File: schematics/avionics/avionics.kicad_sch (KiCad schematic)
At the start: 15 parts, among them SW1 SW_SPST, SW2 SW_DPST, SW3 SW_SPST, SW4 SW_SPST, SW5 SW_DPST, U1 TeleMega

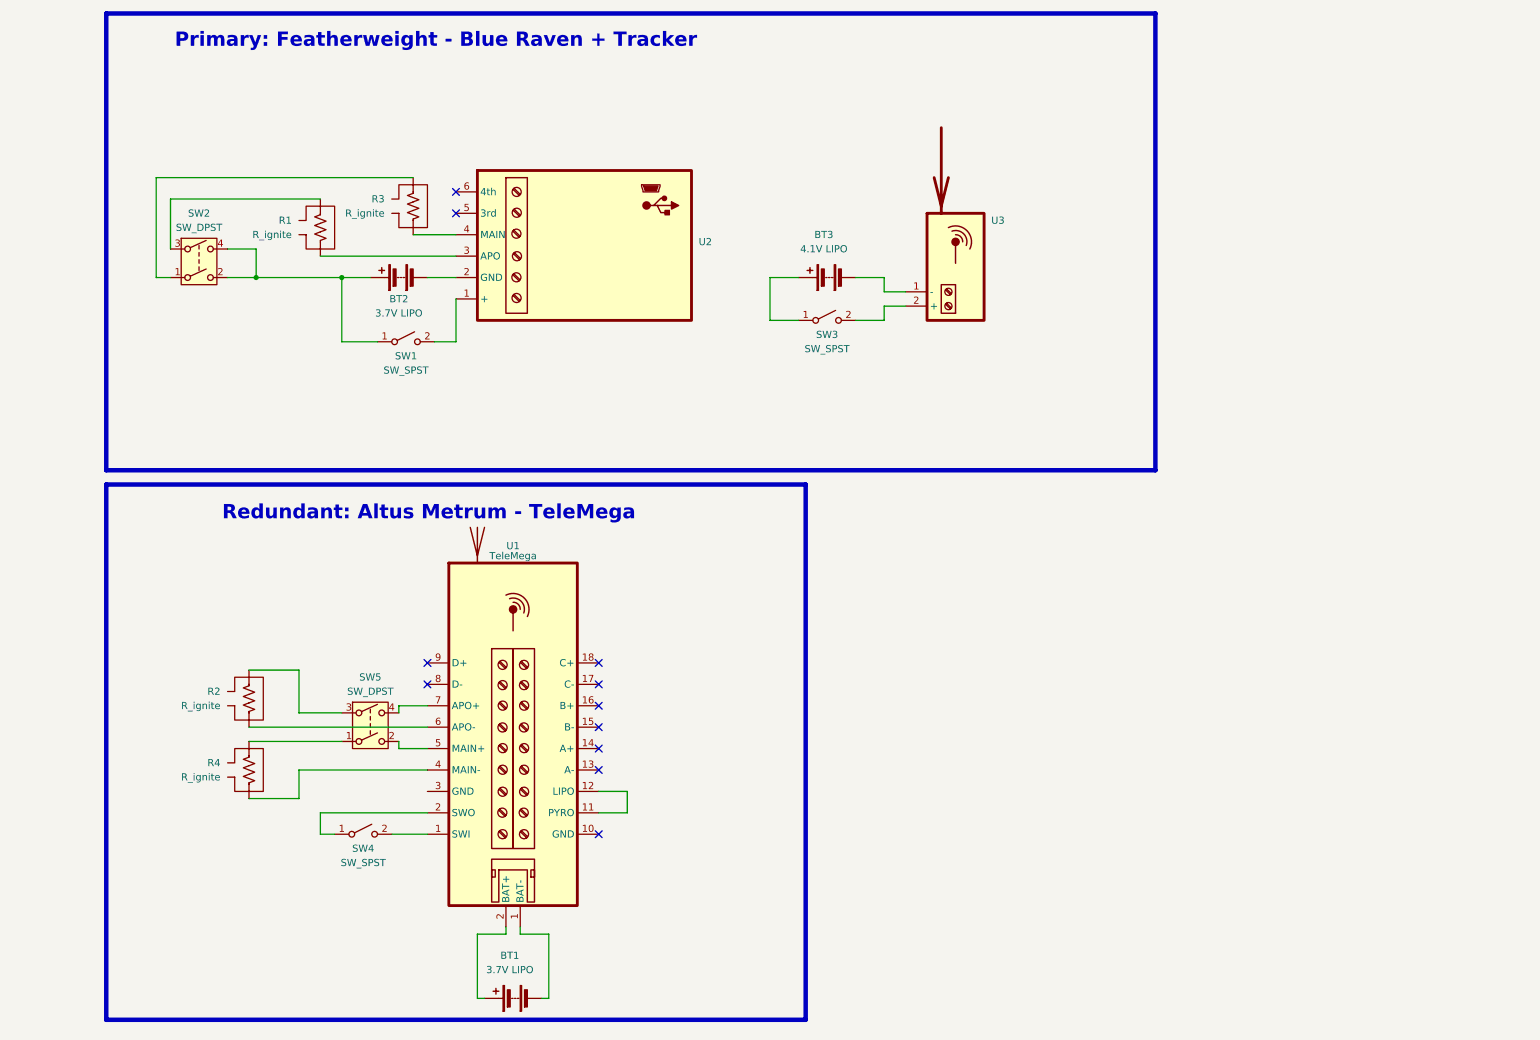
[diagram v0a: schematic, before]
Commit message: updated av bay schematic
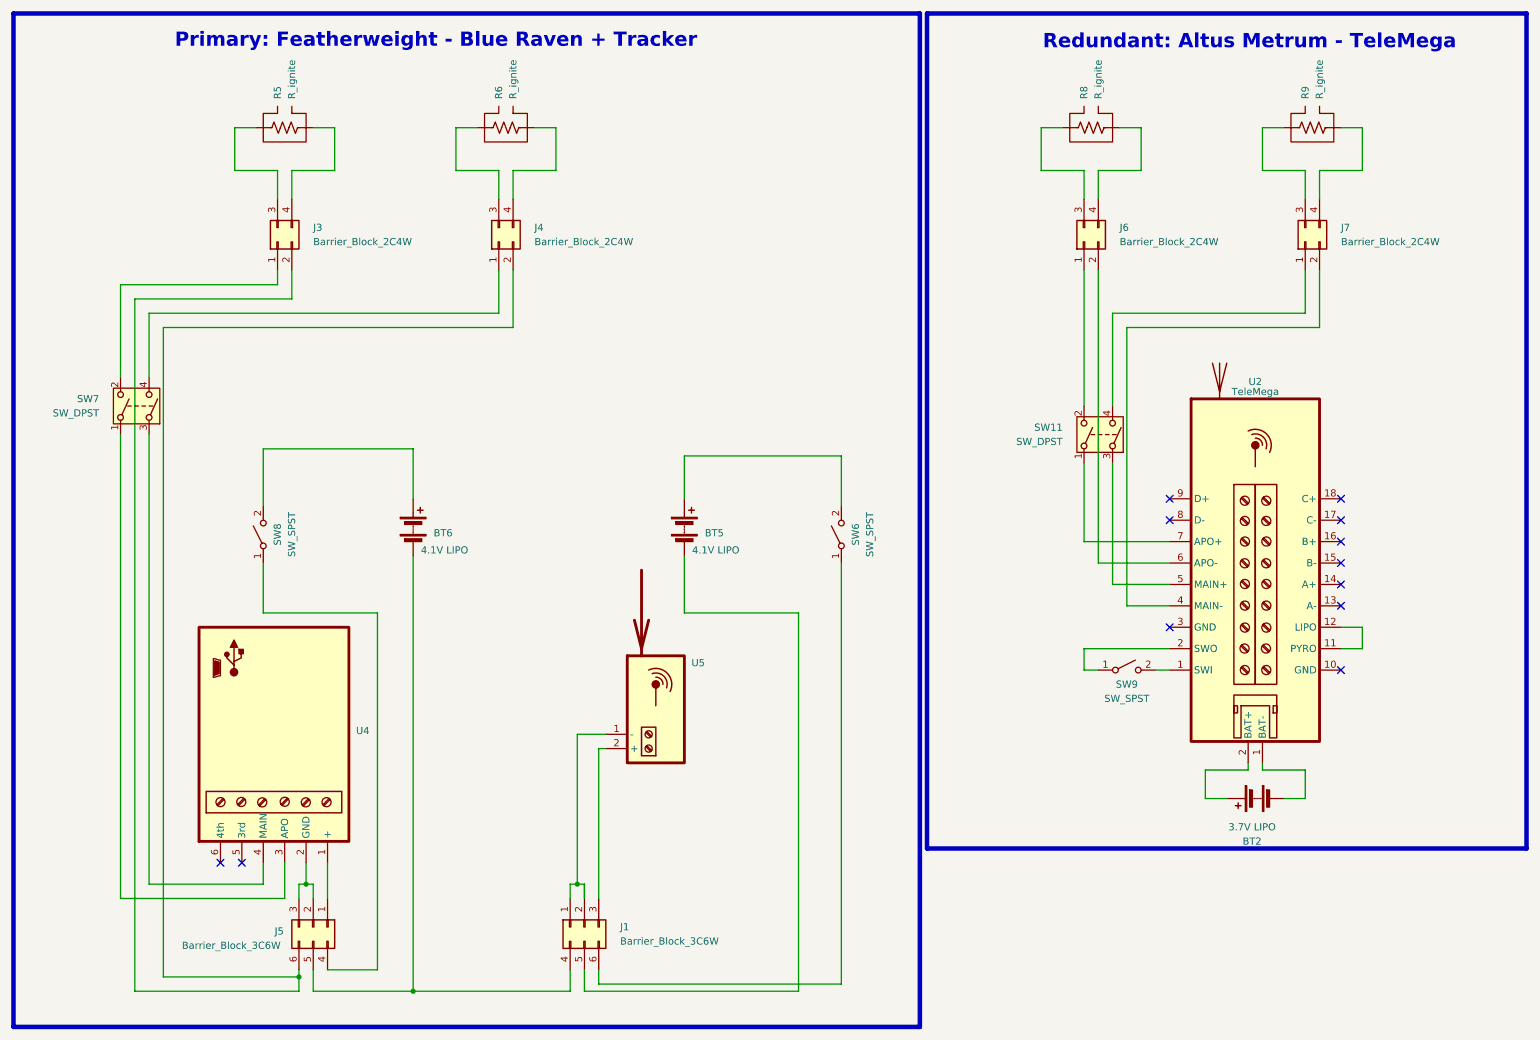
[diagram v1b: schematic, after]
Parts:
- removed BT1: 3.7V LIPO, symbol Device:Battery
- removed BT3: 4.1V LIPO, symbol Device:Battery
- removed R1, R2, R3, R4: R_ignite, symbol recovery:R_Igniter
- removed SW1, SW3, SW4: SW_SPST, symbol Switch:SW_SPST
- removed SW2, SW5: SW_DPST, symbol Switch:SW_DPST
- removed U1: TeleMega, symbol altusmetrum:telemega
- removed U2: ~, symbol featherweight:blue_raven
- removed U3: ~, symbol featherweight:tracker_gps
- added BT5, BT6: 4.1V LIPO, symbol Device:Battery
- added J1, J5: Barrier_Block_3C6W, symbol Connector_Generic:Conn_02x03_Top_Bottom
- added J3, J4, J6, J7: Barrier_Block_2C4W, symbol Connector_Generic:Conn_02x02_Top_Bottom
- added R5, R6, R8, R9: R_ignite, symbol recovery:R_Igniter
- added SW11, SW7: SW_DPST, symbol Switch:SW_DPST
- added SW6, SW8, SW9: SW_SPST, symbol Switch:SW_SPST
- added U2: TeleMega, symbol altusmetrum:telemega
- added U4: ~, symbol featherweight:blue_raven
- added U5: ~, symbol featherweight:tracker_gps
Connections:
- net at BT2.1 (+): now also U2.2 (BAT+)
- net at BT2.2 (-): now also U2.1 (BAT-)
- new net: BT5.1 (+), SW6.2 (B)
- new net: BT5.2 (-), J1.5 (Pin_5)
- new net: SW7.1, U4.3 (APO)
- new net: J3.1 (Pin_1), SW7.2
- new net: SW7.3, U4.4 (MAIN)
- new net: J4.1 (Pin_1), SW7.4
- new net: J3.2 (Pin_2), J4.2 (Pin_2), J5.6 (Pin_6)
- new net: J4.3 (Pin_3), R6.1
- new net: J4.4 (Pin_4), R6.2
- new net: SW9.1 (A), U2.2 (BAT+)
- new net: SW9.2 (B), U2.1 (BAT-)
- new net: J6.1 (Pin_1), SW11.2
- new net: J6.2 (Pin_2), U2.6 (APO-)
- new net: J6.3 (Pin_3), R8.1
- new net: J6.4 (Pin_4), R8.2
- new net: J5.1 (Pin_1), U4.1 (+)
- new net: J5.2 (Pin_2), J5.3 (Pin_3), U4.2 (GND)
- new net: J5.4 (Pin_4), SW8.1 (A)
- new net: BT6.2 (-), J1.4 (Pin_4), J5.5 (Pin_5)
- new net: J7.3 (Pin_3), R9.1
- new net: J7.4 (Pin_4), R9.2
- new net: BT6.1 (+), SW8.2 (B)
- new net: J3.3 (Pin_3), R5.1
- new net: J3.4 (Pin_4), R5.2
- new net: SW11.1, U2.7 (APO+)
- new net: SW11.3, U2.5 (MAIN+)
- new net: J7.1 (Pin_1), SW11.4
- new net: J1.1 (Pin_1), J1.2 (Pin_2), U5.1 (-)
- new net: J1.3 (Pin_3), U5.2 (+)
- new net: J7.2 (Pin_2), U2.4 (MAIN-)
- new net: J1.6 (Pin_6), SW6.1 (A)
- new net: U2.11 (PYRO), U2.12 (LIPO)
- no-connect marks 11 -> 12
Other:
- company: (none) -> WE Rocketry
- title: (none) -> Hyperion2 Avionics Bay Wiring
